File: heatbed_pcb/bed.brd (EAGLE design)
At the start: 34 x 32 mm, 0 parts

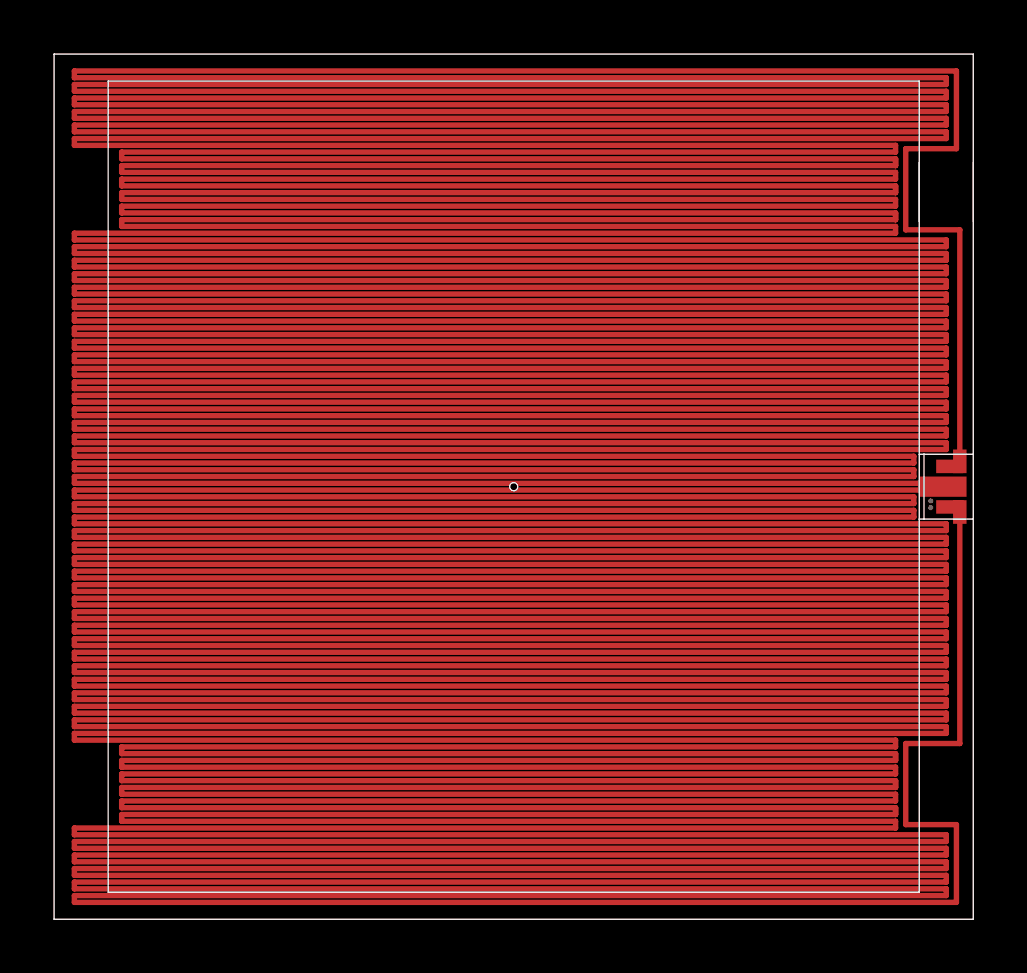
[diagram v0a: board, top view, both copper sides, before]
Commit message: .
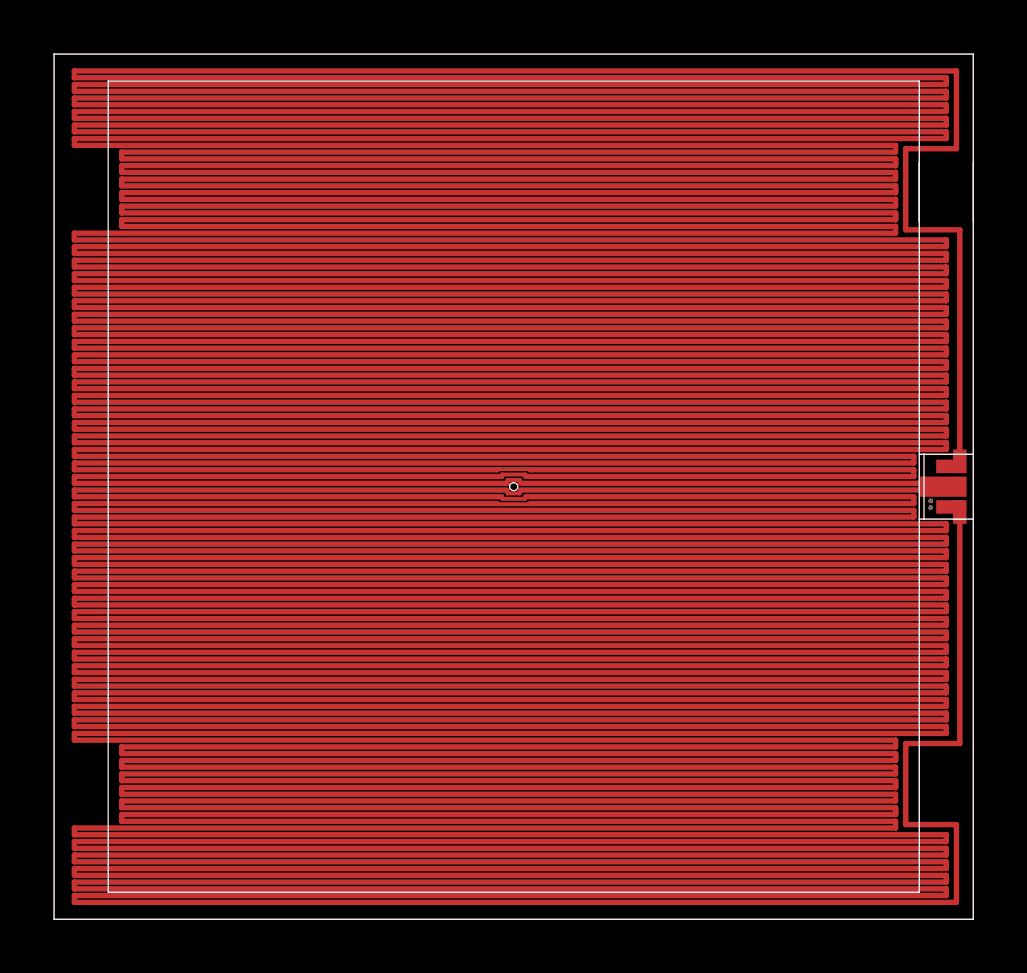
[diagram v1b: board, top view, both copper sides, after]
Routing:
- net S$9: track 352.5 -> 257.9 mm
- net S$25: track 0.00 -> 92.2 mm
- net S$18: track 352.5 -> 348.8 mm
- net S$26: track 0.00 -> 1.35 mm
- net S$30: track 0.00 -> 1.05 mm
- net S$27: track 0.00 -> 1.05 mm
- net S$28: track 0.00 -> 0.73 mm
- net S$29: track 0.00 -> 0.68 mm
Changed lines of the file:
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@@
 <wire x1="33" y1="13.125" x2="0.75" y2="13.125" width="0.2" layer="1"/>
+</signal>
+<signal name="S$23">
+<wire x1="0.75" y1="15.625" x2="0.75" y2="15.875" width="0.2" layer="1"/>
+</signal>
+<signal name="S$24">
+<wire x1="31.8" y1="15.375" x2="31.8" y2="15.625" width="0.2" layer="1"/>
 </signal>
 <signal name="S$9">
@@
 <wire x1="31.8" y1="15.125" x2="0.75" y2="15.125" width="0.2" layer="1"/>
 <wire x1="0.75" y1="15.125" x2="0.75" y2="15.375" width="0.2" layer="1"/>
-<wire x1="0.75" y1="15.375" x2="31.8" y2="15.375" width="0.2" layer="1"/>
-<wire x1="31.8" y1="15.375" x2="31.8" y2="15.625" width="0.2" layer="1"/>
-<wire x1="31.8" y1="15.625" x2="0.75" y2="15.625" width="0.2" layer="1"/>
-<wire x1="0.75" y1="15.625" x2="0.75" y2="15.875" width="0.2" layer="1"/>
-<wire x1="0.75" y1="15.875" x2="32.75" y2="15.875" width="0.2" layer="1"/>
 </signal>
 <signal name="S$10">
@@
 <wire x1="33" y1="18.875" x2="0.75" y2="18.875" width="0.2" layer="1"/>
 </signal>
+<signal name="S$22">
+<wire x1="31.8" y1="16.625" x2="31.8" y2="16.375" width="0.2" layer="1"/>
+</signal>
+<signal name="S$21">
+<wire x1="0.75" y1="16.375" x2="0.75" y2="16.125" width="0.2" layer="1"/>
+</signal>
 <signal name="S$18">
 <wire x1="0.75" y1="18.875" x2="0.75" y2="18.625" width="0.2" layer="1"/>
@@
 <wire x1="31.8" y1="16.875" x2="0.75" y2="16.875" width="0.2" layer="1"/>
 <wire x1="0.75" y1="16.875" x2="0.75" y2="16.625" width="0.2" layer="1"/>
-<wire x1="0.75" y1="16.625" x2="31.8" y2="16.625" width="0.2" layer="1"/>
-<wire x1="31.8" y1="16.625" x2="31.8" y2="16.375" width="0.2" layer="1"/>
-<wire x1="31.8" y1="16.375" x2="0.75" y2="16.375" width="0.2" layer="1"/>
-<wire x1="0.75" y1="16.375" x2="0.75" y2="16.125" width="0.2" layer="1"/>
-<wire x1="0.75" y1="16.125" x2="32.75" y2="16.125" width="0.2" layer="1"/>
+<wire x1="16.4" y1="16.625" x2="0.75" y2="16.625" width="0.2" layer="1"/>
+<wire x1="16.55" y1="16.375" x2="0.75" y2="16.375" width="0.2" layer="1"/>
+<wire x1="16.75" y1="16.125" x2="0.75" y2="16.125" width="0.2" layer="1"/>
+<wire x1="17.25" y1="16.125" x2="32.15" y2="16.125" width="0.2" layer="1"/>
+<wire x1="17.45" y1="16.375" x2="31.8" y2="16.375" width="0.2" layer="1"/>
+<wire x1="17.6" y1="16.625" x2="31.8" y2="16.625" width="0.2" layer="1"/>
 </signal>
 <signal name="S$19">
@@
 <via x="32.425" y="15.225" extent="1-16" drill="0.01" diameter="0.2" shape="square"/>
 </signal>
+<signal name="S$25">
+<wire x1="16.4" y1="15.375" x2="0.75" y2="15.375" width="0.2" layer="1"/>
+<wire x1="16.55" y1="15.625" x2="0.75" y2="15.625" width="0.2" layer="1"/>
+<wire x1="16.75" y1="15.875" x2="0.75" y2="15.875" width="0.2" layer="1"/>
+<wire x1="17.25" y1="15.875" x2="32.15" y2="15.875" width="0.2" layer="1"/>
+<wire x1="17.45" y1="15.625" x2="31.8" y2="15.625" width="0.2" layer="1"/>
+<wire x1="17.6" y1="15.375" x2="31.8" y2="15.375" width="0.2" layer="1"/>
+<wire x1="16.4" y1="15.375" x2="16.4" y2="15.35" width="0.15" layer="1"/>
+<wire x1="16.4" y1="15.35" x2="17.625" y2="15.35" width="0.15" layer="1"/>
+</signal>
+<signal name="S$26">
+<wire x1="16.4" y1="16.6" x2="16.4" y2="16.65" width="0.15" layer="1"/>
+<wire x1="16.4" y1="16.65" x2="17.65" y2="16.65" width="0.15" layer="1"/>
+<wire x1="17.65" y1="16.65" x2="17.65" y2="16.6" width="0.15" layer="1"/>
+</signal>
+<signal name="S$27">
+<wire x1="16.575" y1="16.35" x2="16.575" y2="16.45" width="0.15" layer="1"/>
+<wire x1="16.575" y1="16.45" x2="17.425" y2="16.45" width="0.15" layer="1"/>
+<wire x1="17.425" y1="16.45" x2="17.425" y2="16.35" width="0.15" layer="1"/>
+</signal>
+<signal name="S$28">
+<wire x1="16.775" y1="16.1" x2="16.775" y2="16.25" width="0.15" layer="1"/>
+<wire x1="16.775" y1="16.25" x2="17.225" y2="16.25" width="0.15" layer="1"/>
+<wire x1="17.225" y1="16.25" x2="17.225" y2="16.125" width="0.15" layer="1"/>
+</signal>
+<signal name="S$29">
+<wire x1="17.225" y1="15.875" x2="17.225" y2="15.75" width="0.15" layer="1"/>
+<wire x1="17.225" y1="15.75" x2="16.775" y2="15.75" width="0.15" layer="1"/>
+<wire x1="16.775" y1="15.75" x2="16.775" y2="15.85" width="0.15" layer="1"/>
+</signal>
+<signal name="S$30">
+<wire x1="16.575" y1="15.65" x2="16.575" y2="15.55" width="0.15" layer="1"/>
+<wire x1="16.575" y1="15.55" x2="17.425" y2="15.55" width="0.15" layer="1"/>
+<wire x1="17.425" y1="15.55" x2="17.425" y2="15.65" width="0.15" layer="1"/>
+</signal>
 </signals>
